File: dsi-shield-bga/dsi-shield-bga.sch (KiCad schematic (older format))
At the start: 0 parts

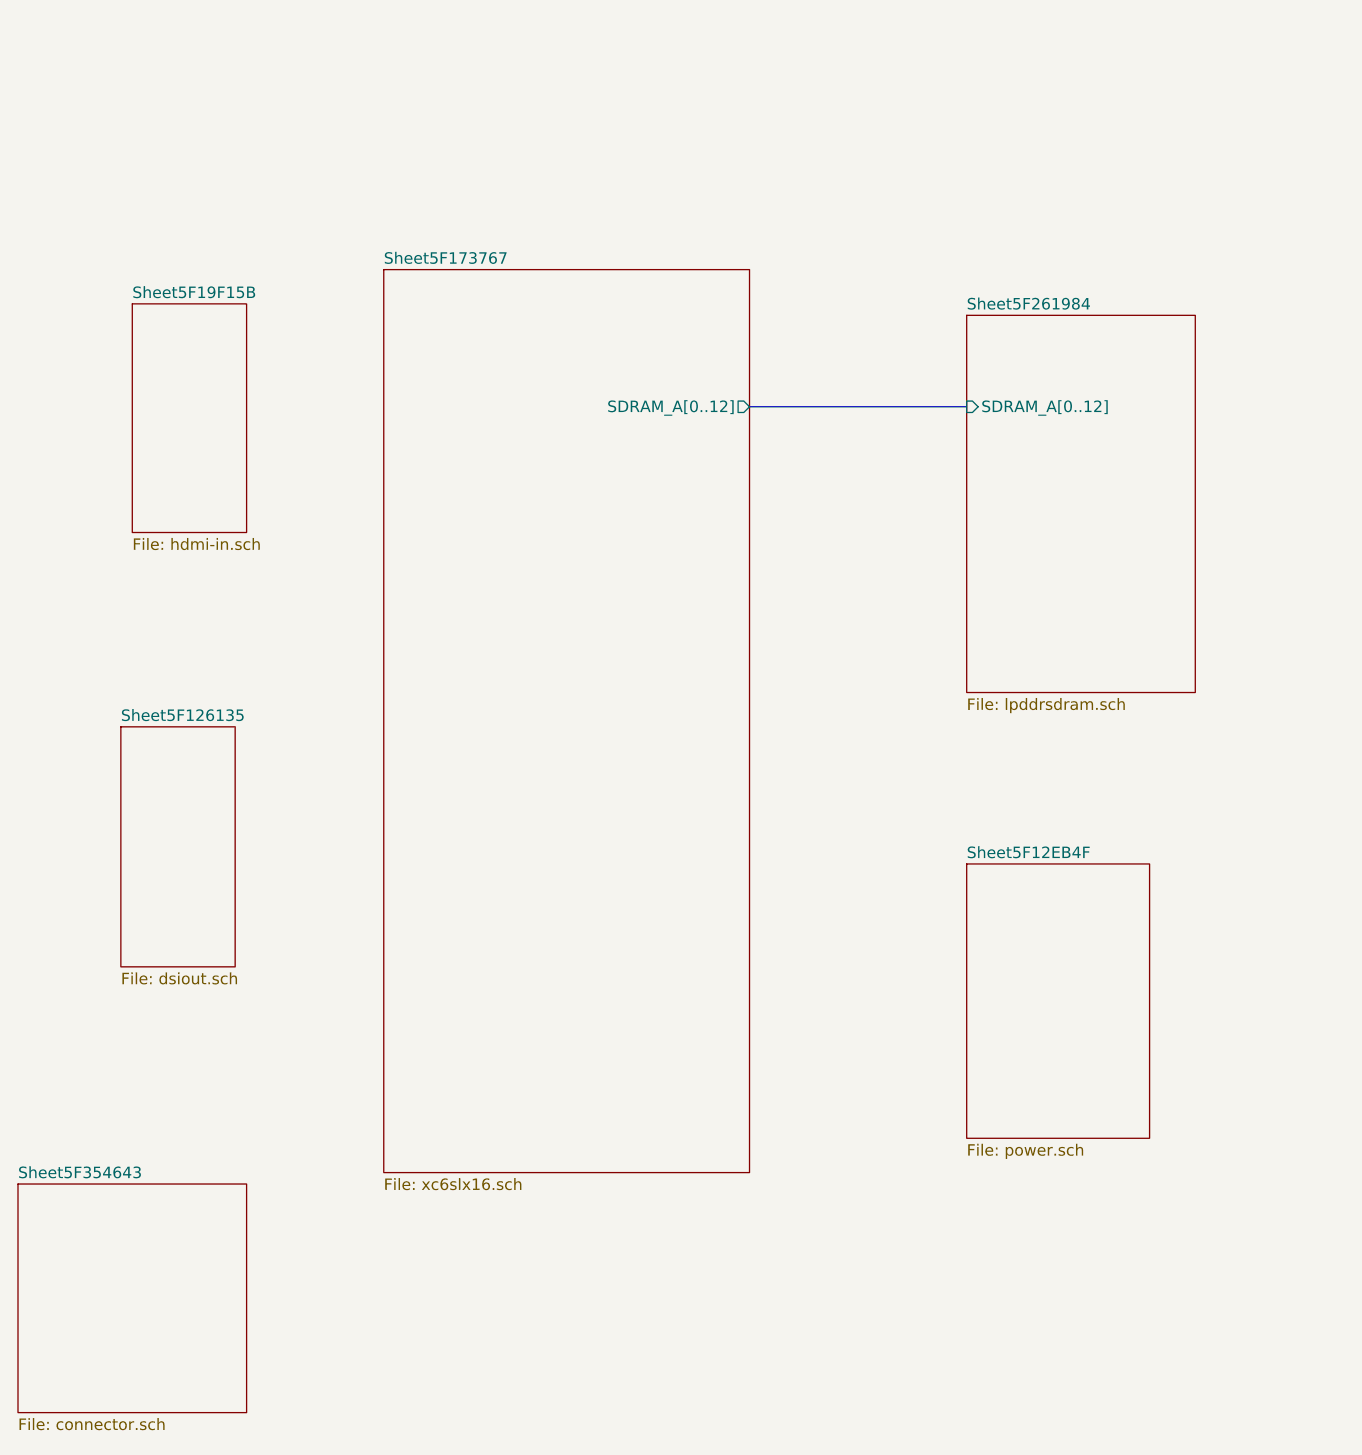
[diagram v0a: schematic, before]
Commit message: 20200808
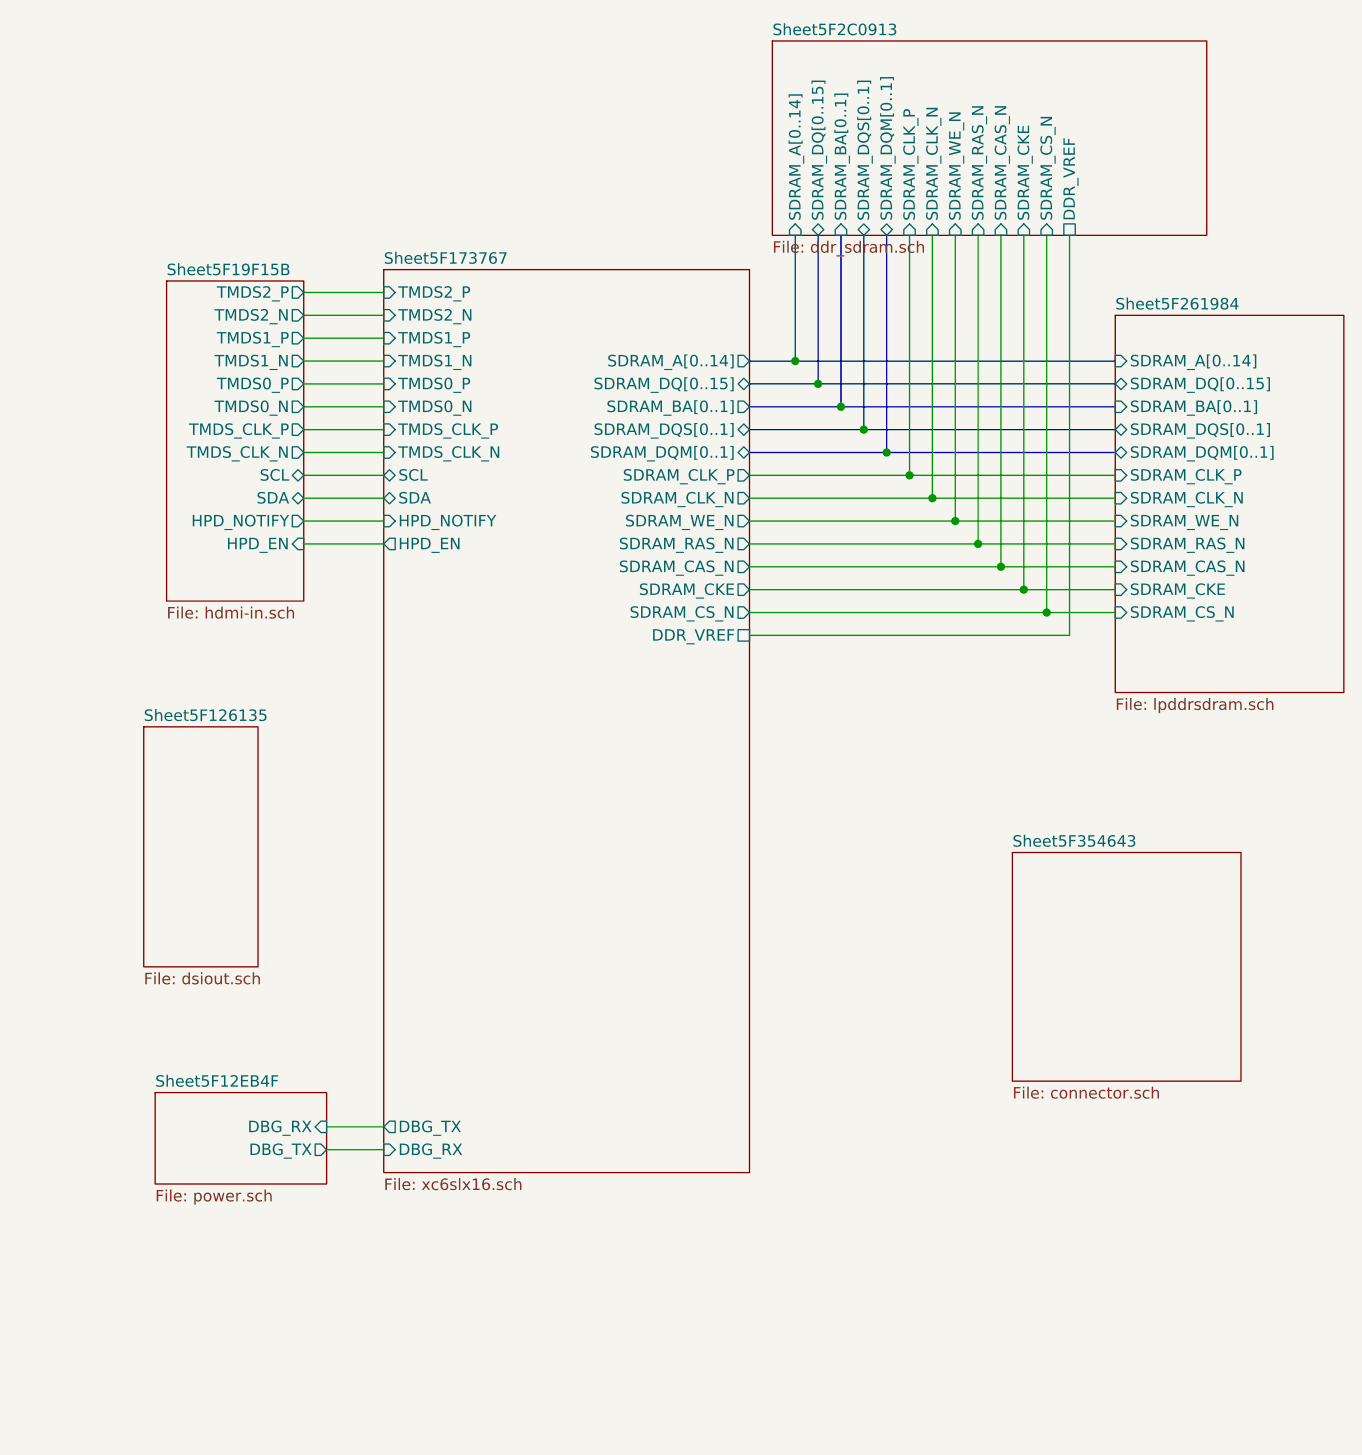
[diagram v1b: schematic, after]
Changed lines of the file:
@@
 $Descr A4 11693 8268
 encoding utf-8
-Sheet 1 7
+Sheet 1 8
 Title "xc6slx16"
 Date ""
@@
 Comment4 ""
 $EndDescr
-Wire Bus Line
-	7300 2500 8250 2500
+$Sheet
+S 4750 1950 600  1400
+U 5F19F15C
+F0 "Sheet5F19F15B" 50
+F1 "hdmi-in.sch" 50
+F2 "TMDS2_P" O R 5350 2000 50
+F3 "TMDS2_N" O R 5350 2100 50
+F4 "TMDS1_P" O R 5350 2200 50
+F5 "TMDS1_N" O R 5350 2300 50
+F6 "TMDS0_P" O R 5350 2400 50
+F7 "TMDS0_N" O R 5350 2500 50
+F8 "TMDS_CLK_P" O R 5350 2600 50
+F9 "TMDS_CLK_N" O R 5350 2700 50
+F10 "SCL" B R 5350 2800 50
+F11 "SDA" B R 5350 2900 50
+F12 "HPD_NOTIFY" O R 5350 3000 50
+F13 "HPD_EN" I R 5350 3100 50
+$EndSheet
+$Sheet
+S 4650 3900 500  1050
+U 5F126136
+F0 "Sheet5F126135" 50
+F1 "dsiout.sch" 50
+$EndSheet
+$Sheet
+S 4700 5500 750  400
+U 5F12EB50
+F0 "Sheet5F12EB4F" 50
+F1 "power.sch" 50
+F2 "DBG_RX" I R 5450 5650 50
+F3 "DBG_TX" O R 5450 5750 50
+$EndSheet
+$Sheet
+S 8450 4450 1000 1000
+U 5F354644
+F0 "Sheet5F354643" 50
+F1 "connector.sch" 50
+$EndSheet
+Wire Bus Line
+	7300 2300 7500 2300
+Wire Bus Line
+	8900 2400 7600 2400
+Wire Bus Line
+	7300 2500 7700 2500
+Wire Bus Line
+	8900 2600 7800 2600
+Wire Bus Line
+	7300 2700 7900 2700
+Wire Wire Line
+	8900 2800 8000 2800
+Wire Wire Line
+	7300 2900 8100 2900
+Wire Wire Line
+	8900 3000 8200 3000
+Wire Wire Line
+	7300 3100 8300 3100
+Wire Wire Line
+	8900 3200 8400 3200
+Wire Wire Line
+	7300 3300 8500 3300
+Wire Wire Line
+	8900 3400 8600 3400
+Wire Wire Line
+	5350 2000 5700 2000
+Wire Wire Line
+	5350 2100 5700 2100
+Wire Wire Line
+	5350 2200 5700 2200
+Wire Wire Line
+	5350 2300 5700 2300
+Wire Wire Line
+	5350 2400 5700 2400
+Wire Wire Line
+	5350 2500 5700 2500
+Wire Wire Line
+	5350 2600 5700 2600
+Wire Wire Line
+	5350 2700 5700 2700
+Wire Wire Line
+	5350 2800 5700 2800
+Wire Wire Line
+	5350 2900 5700 2900
+Wire Wire Line
+	5350 3000 5700 3000
+Wire Wire Line
+	5350 3100 5700 3100
+Wire Wire Line
+	5450 5650 5700 5650
+Wire Wire Line
+	5450 5750 5700 5750
+$Sheet
+S 8900 2100 1000 1650
+U 5F261985
+F0 "Sheet5F261984" 50
+F1 "lpddrsdram.sch" 50
+F2 "SDRAM_A[0..14]" I L 8900 2300 50
+F3 "SDRAM_DQ[0..15]" B L 8900 2400 50
+F4 "SDRAM_BA[0..1]" I L 8900 2500 50
+F5 "SDRAM_DQS[0..1]" B L 8900 2600 50
+F6 "SDRAM_DQM[0..1]" B L 8900 2700 50
+F7 "SDRAM_CLK_P" I L 8900 2800 50
+F8 "SDRAM_CLK_N" I L 8900 2900 50
+F9 "SDRAM_WE_N" I L 8900 3000 50
+F10 "SDRAM_RAS_N" I L 8900 3100 50
+F11 "SDRAM_CAS_N" I L 8900 3200 50
+F12 "SDRAM_CKE" I L 8900 3300 50
+F13 "SDRAM_CS_N" I L 8900 3400 50
+$EndSheet
+Connection ~ 7500 2300
+Wire Bus Line
+	7500 2300 8900 2300
+Connection ~ 7600 2400
+Wire Bus Line
+	7600 2400 7300 2400
+Connection ~ 7700 2500
+Wire Bus Line
+	7700 2500 8900 2500
+Connection ~ 7800 2600
+Wire Bus Line
+	7800 2600 7300 2600
+Connection ~ 7900 2700
+Wire Bus Line
+	7900 2700 8900 2700
+Connection ~ 8000 2800
+Wire Wire Line
+	8000 2800 7300 2800
+Connection ~ 8100 2900
+Wire Wire Line
+	8100 2900 8900 2900
+Connection ~ 8200 3000
+Wire Wire Line
+	8200 3000 7300 3000
+Connection ~ 8300 3100
+Wire Wire Line
+	8300 3100 8900 3100
+Connection ~ 8400 3200
+Wire Wire Line
+	8400 3200 7300 3200
+Connection ~ 8500 3300
+Wire Wire Line
+	8500 3300 8900 3300
+Connection ~ 8600 3400
+Wire Wire Line
+	8600 3400 7300 3400
+Wire Bus Line
+	7800 1750 7800 2600
+Wire Bus Line
+	7900 1750 7900 2700
+Wire Bus Line
+	7600 1750 7600 2400
+Wire Wire Line
+	8100 1750 8100 2900
+Wire Wire Line
+	8000 1750 8000 2800
+Wire Wire Line
+	8500 1750 8500 3300
+Wire Wire Line
+	8600 1750 8600 3400
+Wire Wire Line
+	8200 1750 8200 3000
+Wire Wire Line
+	8400 1750 8400 3200
+Wire Wire Line
+	8300 1750 8300 3100
+Wire Bus Line
+	7700 1750 7700 2500
+Wire Bus Line
+	7500 1750 7500 2300
+$Sheet
+S 7400 900  1900 850
+U 5F2C0914
+F0 "Sheet5F2C0913" 50
+F1 "ddr_sdram.sch" 50
+F2 "SDRAM_A[0..14]" I B 7500 1750 50
+F3 "SDRAM_BA[0..1]" I B 7700 1750 50
+F4 "SDRAM_RAS_N" I B 8300 1750 50
+F5 "SDRAM_CAS_N" I B 8400 1750 50
+F6 "SDRAM_WE_N" I B 8200 1750 50
+F7 "SDRAM_CS_N" I B 8600 1750 50
+F8 "SDRAM_CKE" I B 8500 1750 50
+F9 "SDRAM_CLK_P" I B 8000 1750 50
+F10 "SDRAM_CLK_N" I B 8100 1750 50
+F11 "SDRAM_DQ[0..15]" B B 7600 1750 50
+F12 "SDRAM_DQM[0..1]" B B 7900 1750 50
+F13 "SDRAM_DQS[0..1]" B B 7800 1750 50
+F14 "DDR_VREF" U B 8700 1750 50
+$EndSheet
 $Sheet
 S 5700 1900 1600 3950
@@
 F0 "Sheet5F173767" 50
 F1 "xc6slx16.sch" 50
-F2 "SDRAM_A[0..12]" O R 7300 2500 50
-$EndSheet
-$Sheet
-S 8250 2100 1000 1650
-U 5F261985
-F0 "Sheet5F261984" 50
-F1 "lpddrsdram.sch" 50
-F2 "SDRAM_A[0..12]" I L 8250 2500 50
-$EndSheet
-$Sheet
-S 4600 2050 500  1000
-U 5F19F15C
-F0 "Sheet5F19F15B" 50
-F1 "hdmi-in.sch" 50
-$EndSheet
-$Sheet
-S 4550 3900 500  1050
-U 5F126136
-F0 "Sheet5F126135" 50
-F1 "dsiout.sch" 50
-$EndSheet
-$Sheet
-S 8250 4500 800  1200
-U 5F12EB50
-F0 "Sheet5F12EB4F" 50
-F1 "power.sch" 50
-$EndSheet
-$Sheet
-S 4100 5900 1000 1000
-U 5F354644
-F0 "Sheet5F354643" 50
-F1 "connector.sch" 50
-$EndSheet
+F2 "SDRAM_A[0..14]" O R 7300 2300 50
+F3 "SDRAM_DQ[0..15]" B R 7300 2400 50
+F4 "SDRAM_BA[0..1]" O R 7300 2500 50
+F5 "SDRAM_DQS[0..1]" B R 7300 2600 50
+F6 "SDRAM_DQM[0..1]" B R 7300 2700 50
+F7 "SDRAM_CLK_P" O R 7300 2800 50
+F8 "SDRAM_CLK_N" O R 7300 2900 50
+F9 "SDRAM_WE_N" O R 7300 3000 50
+F10 "SDRAM_RAS_N" O R 7300 3100 50
+F11 "SDRAM_CAS_N" O R 7300 3200 50
+F12 "SDRAM_CKE" O R 7300 3300 50
+F13 "SDRAM_CS_N" O R 7300 3400 50
+F14 "HPD_NOTIFY" I L 5700 3000 50
+F15 "TMDS0_P" I L 5700 2400 50
+F16 "TMDS0_N" I L 5700 2500 50
+F17 "TMDS1_P" I L 5700 2200 50
+F18 "TMDS1_N" I L 5700 2300 50
+F19 "TMDS2_P" I L 5700 2000 50
+F20 "TMDS2_N" I L 5700 2100 50
+F21 "TMDS_CLK_P" I L 5700 2600 50
+F22 "TMDS_CLK_N" I L 5700 2700 50
+F23 "SCL" B L 5700 2800 50
+F24 "SDA" B L 5700 2900 50
+F25 "HPD_EN" O L 5700 3100 50
+F26 "DBG_TX" O L 5700 5650 50
+F27 "DBG_RX" I L 5700 5750 50
+F28 "DDR_VREF" U R 7300 3500 50
+$EndSheet
+Wire Wire Line
+	8700 1750 8700 3500
+Wire Wire Line
+	8700 3500 7300 3500
 $EndSCHEMATC
